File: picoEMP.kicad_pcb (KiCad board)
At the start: 2 copper layers, 101 x 43 mm, 41 parts, among them J1 Conn_01x02, J2 Conn_Coaxial, J3 Conn_01x07, J4 Conn_01x02, J5 Conn_01x02, J6 Conn_01x04, Q1 AO3422, Q2 AO3422, Q3 RGT16BM65DTL, SW1 SW_Push, SW2 SW_Push, SW3 SW_Push, T1 PE-68386NL, T2 PE-68386NL, U1 SFH601-2X007

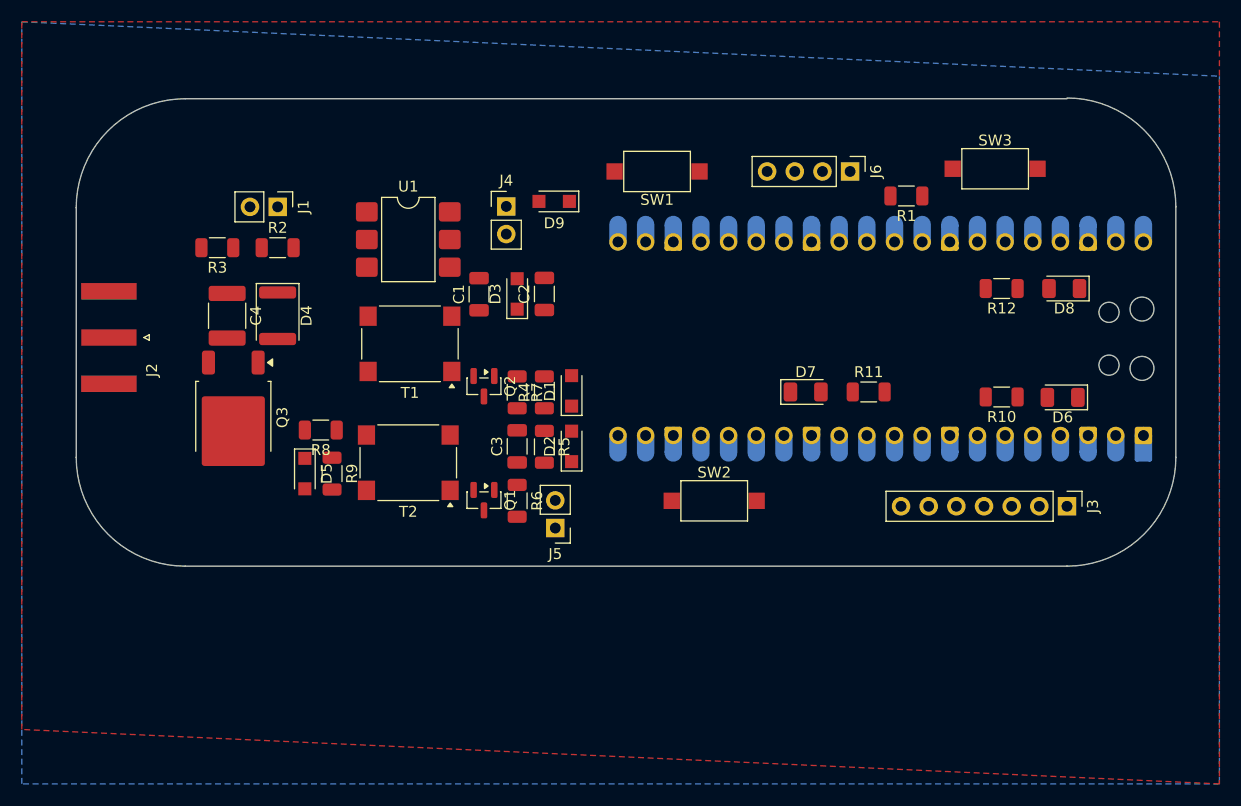
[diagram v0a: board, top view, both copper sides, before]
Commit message: 'pads_añadidos'
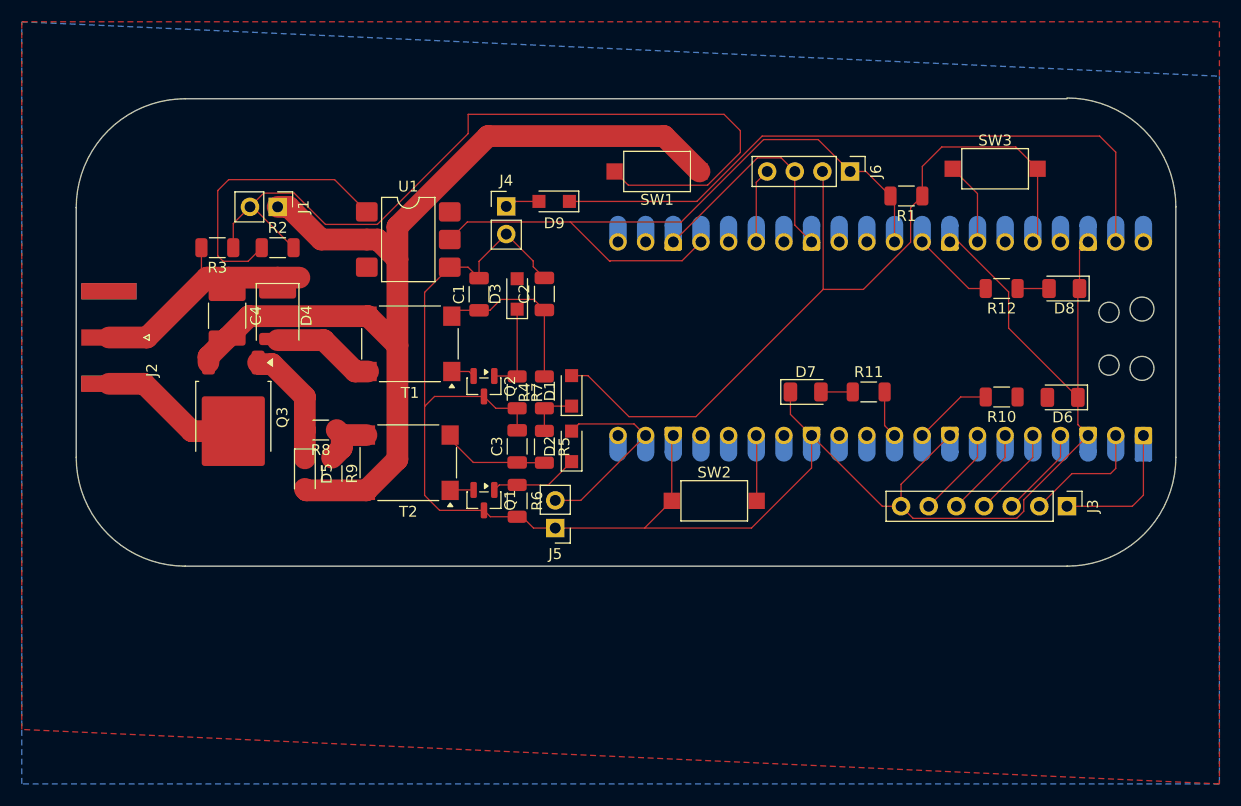
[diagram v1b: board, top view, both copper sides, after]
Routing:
- net GND: track 0.00 -> 204.2 mm
- net Net-(D5-A): track 0.00 -> 97.2 mm
- net Net-(J1-Pin_2): track 0.00 -> 77.9 mm
- net VCC: track 0.00 -> 76.7 mm
- net CHARGED: track 0.00 -> 65.0 mm
- net Net-(A1-VSYS): track 0.00 -> 61.5 mm
- net Net-(R2-Pad1): track 0.00 -> 26.1 mm
- net Net-(D4-K): track 0.00 -> 25.6 mm
- net HVPULSE: track 0.00 -> 18.3 mm
- net Net-(C1-Pad1): track 0.00 -> 15.6 mm
- net Net-(J2-Ext): track 0.00 -> 13.2 mm
- net Net-(A1-GPIO0): track 0.00 -> 12.9 mm
- net Net-(A1-GPIO1): track 0.00 -> 11.5 mm
- net Net-(D5-K): track 0.00 -> 11.3 mm
- net Net-(C3-Pad1): track 0.00 -> 9.93 mm
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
